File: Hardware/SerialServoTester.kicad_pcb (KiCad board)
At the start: 2 copper layers, 0 parts

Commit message: Update PCB data
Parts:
- added J1: Conn_01x04_Pin, Connector_PinHeader_2.54mm:PinHeader_1x04_P2.54mm_Horizontal, F.Cu at (133.6, 72.4)
- added J2: Screw_Terminal_01x02, TerminalBlock:TerminalBlock_bornier-2_P5.08mm, F.Cu at (123.5, 70.0)
- added P1: USB_C_Plug_USB2.0, Connector_USB:USB_C_Plug_JAE_DX07P024AJ1, F.Cu at (109.0, 77.0)
- added Q1: BSS84, Package_TO_SOT_SMD:SOT-23, F.Cu at (114.9, 72.0)
- added R1: 5.1k, Resistor_SMD:R_0603_1608Metric_Pad0.98x0.95mm_HandSolder, F.Cu at (114.0, 78.0)
- added R2: 5.1k, Resistor_SMD:R_0603_1608Metric_Pad0.98x0.95mm_HandSolder, F.Cu at (120.0, 78.0)
- added R3: 5.1k, Resistor_SMD:R_0603_1608Metric_Pad0.98x0.95mm_HandSolder, F.Cu at (118.0, 72.0)
- added R4: 5.1k, Resistor_SMD:R_0603_1608Metric_Pad0.98x0.95mm_HandSolder, F.Cu at (120.0, 72.1)
- added R5: 5.1k, Resistor_SMD:R_0603_1608Metric_Pad0.98x0.95mm_HandSolder, F.Cu at (118.0, 78.0)
- added R6: 5.1k, Resistor_SMD:R_0603_1608Metric_Pad0.98x0.95mm_HandSolder, F.Cu at (116.0, 78.1)
- added U1: FT230XS, Package_SO:SSOP-16_3.9x4.9mm_P0.635mm, F.Cu at (117.0, 83.0)
- added U2: LT1785AxN8, Package_DIP:DIP-8_W7.62mm, F.Cu at (122.2, 76.2)
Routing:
- net GND: track 0.00 -> 89.1 mm, vias 0 -> 9
- net VCC: track 0.00 -> 65.1 mm, vias 0 -> 3
- net Net-(J1-Pin_4): track 0.00 -> 35.8 mm
- net Net-(U1-TXD): track 0.00 -> 23.3 mm, vias 0 -> 2
- net Net-(P1-D-): track 0.00 -> 21.8 mm
- net Net-(J1-Pin_3): track 0.00 -> 21.3 mm, vias 0 -> 1
- net Net-(U1-RXD): track 0.00 -> 20.9 mm, vias 0 -> 2
- net Net-(P1-CC): track 0.00 -> 20.5 mm
- net Net-(P1-D+): track 0.00 -> 18.7 mm, vias 0 -> 2
- net Net-(U1-CBUS0): track 0.00 -> 17.0 mm, vias 0 -> 2
- net Net-(J1-Pin_2): track 0.00 -> 15.8 mm
- net /~{EN_4PIN}: track 0.00 -> 14.8 mm, vias 0 -> 4
- net Net-(Q1-D): track 0.00 -> 2.76 mm
- added copper zone on B.Cu, net GND
- added copper zone on F.Cu, net VCC
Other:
- board outline added: 39 x 22 mm

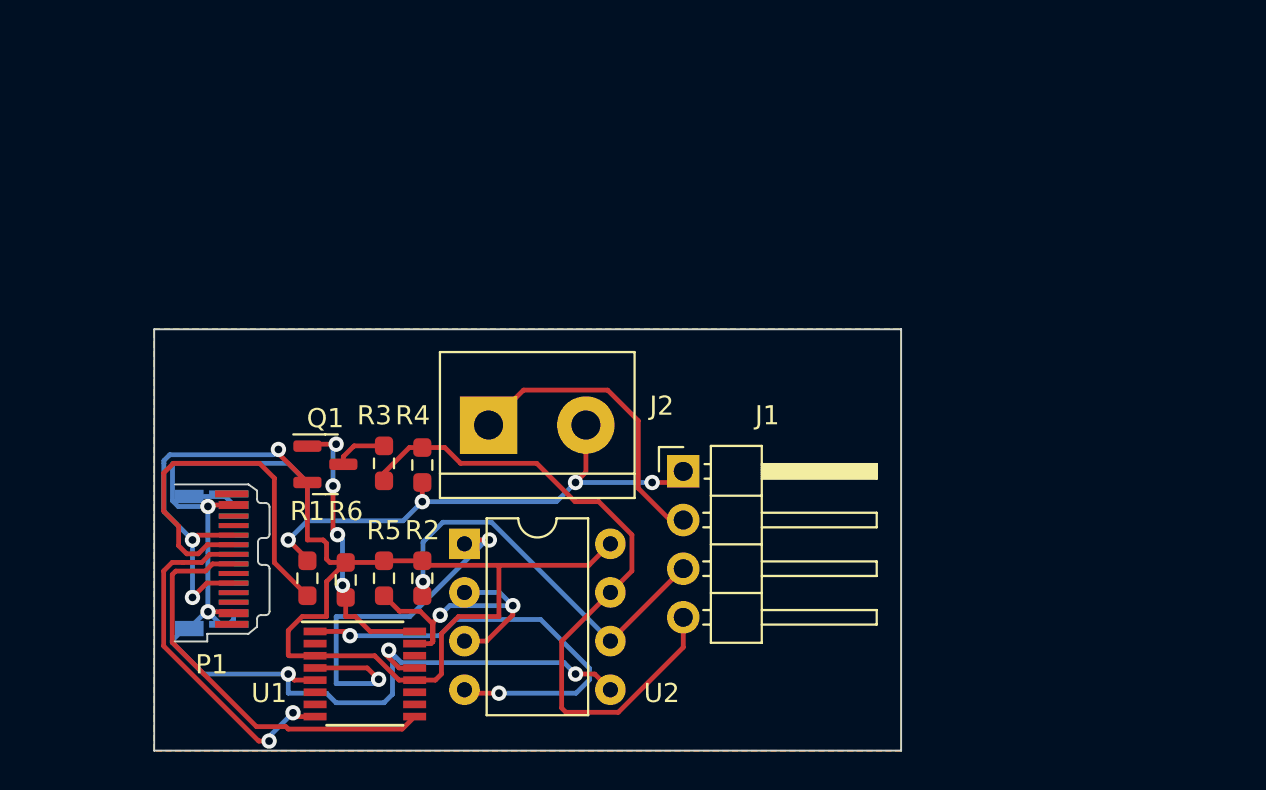
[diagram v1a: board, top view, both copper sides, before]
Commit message: Update PCB design
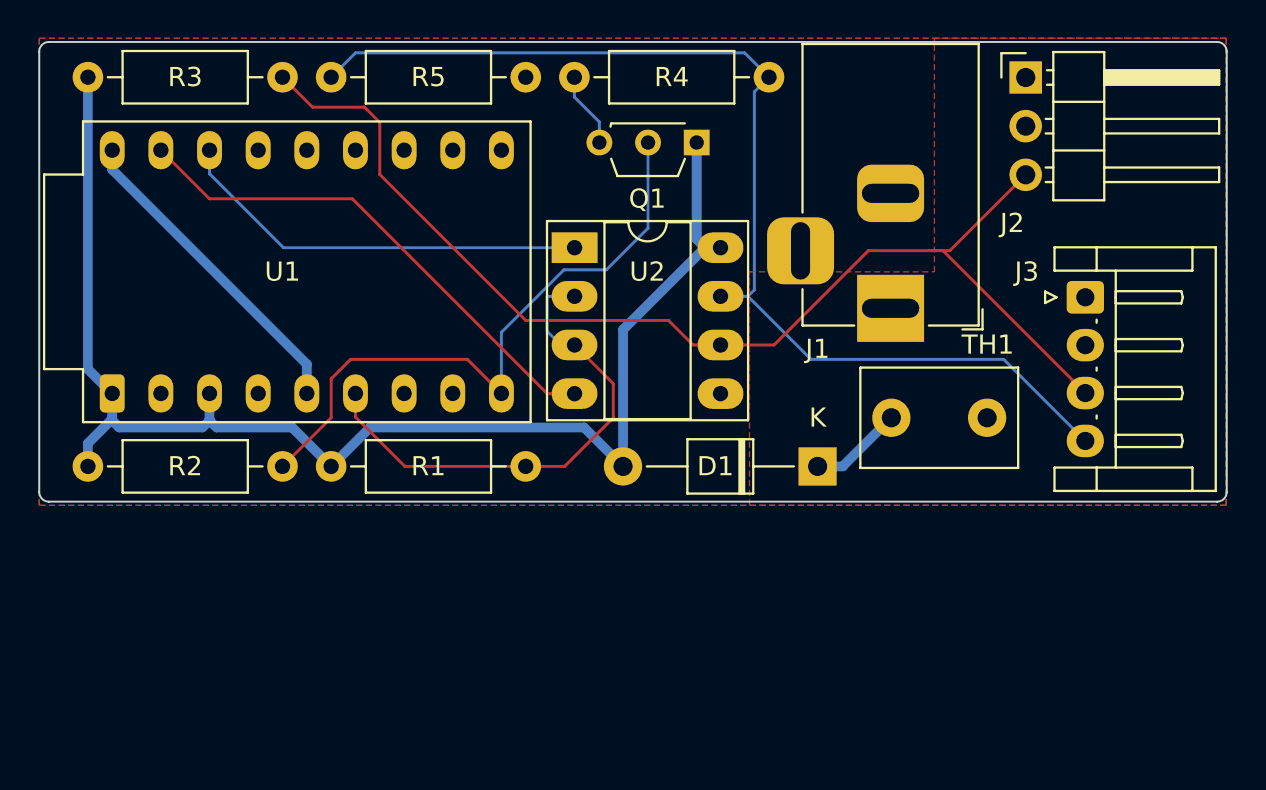
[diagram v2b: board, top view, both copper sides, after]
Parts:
- removed P1: USB_C_Plug_USB2.0, Connector_USB:USB_C_Plug_JAE_DX07P024AJ1
- removed R6: 5.1k, Resistor_SMD:R_0603_1608Metric_Pad0.98x0.95mm_HandSolder
- added D1: 11EQS03L, Diode_THT:D_T-1_P10.16mm_Horizontal, F.Cu at (140.6, 72.2)
- added J3: Conn_01x04_Pin, Connector_JST:JST_EH_S4B-EH_1x04_P2.50mm_Horizontal, F.Cu at (154.6, 63.3)
- added TH1: PTGL07AR820M9A51B0, Capacitor_THT:C_Disc_D8.0mm_W5.0mm_P5.00mm, F.Cu at (149.5, 69.6)
- J1: value Conn_01x04_Pin -> MJ-179PH; footprint Connector_PinHeader_2.54mm:PinHeader_1x04_P2.54mm_Horizontal -> Connector_BarrelJack:BarrelJack_Horizontal
- J2: value Screw_Terminal_01x02 -> Conn_01x03_Pin; footprint TerminalBlock:TerminalBlock_bornier-2_P5.08mm -> Connector_PinHeader_2.54mm:PinHeader_1x03_P2.54mm_Horizontal
- Q1: value BSS84 -> 2SJ498-D; footprint Package_TO_SOT_SMD:SOT-23 -> Package_TO_SOT_THT:TO-92S_Wide
- R1, R2, R3, R4, R5: footprint Resistor_SMD:R_0603_1608Metric_Pad0.98x0.95mm_HandSolder -> Resistor_THT:R_Axial_DIN0207_L6.3mm_D2.5mm_P10.16mm_Horizontal
- U1: value FT230XS -> FT231XS_Breakout; footprint Package_SO:SSOP-16_3.9x4.9mm_P0.635mm -> FootprintLibrary:DIP-18_500_ELL
- U2: footprint Package_DIP:DIP-8_W7.62mm -> Package_DIP:DIP-8_W7.62mm_Socket_LongPads
- moved J2 33.4 mm to (151.5, 51.9)
- moved R5 27.2 mm to (125.4, 51.8), turned to 180 degrees
- moved R4 27.2 mm to (138.1, 51.8), turned to 180 degrees
- moved Q1 25.7 mm to (134.3, 55.2), turned to 180 degrees
- moved U1 21.2 mm to (114.0, 62.0)
- moved R3 20.8 mm to (112.7, 51.8), turned to 180 degrees
- moved U2 16.5 mm to (128.0, 60.7)
- moved J1 13.8 mm to (144.4, 63.9), turned to -90 degrees
- moved R1 12.8 mm to (125.4, 72.2), turned to 180 degrees
- moved R2 9.35 mm to (112.7, 72.2), turned to 180 degrees
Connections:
- J1 pad 1: GND -> VCC
- J1 pad 2: Net-(J1-Pin_2) -> GND
- J1 pad 3: Net-(J1-Pin_3) -> GND
- J2 pad 1: Net-(J1-Pin_2) -> GND
- J2 pad 2: GND -> VCC
- Q1 pad 1: /~{EN_4PIN} -> Net-(D1-A)
- Q1 pad 2: VCC -> /~{EN_4PIN}
- Q1 pad 3: Net-(Q1-D) -> Net-(Q1-S)
- R1 pad 1: Net-(P1-CC) -> Net-(U1-CBUS0)
- R1 pad 2: GND -> Net-(D1-A)
- R2 pad 1: Net-(J1-Pin_3) -> /~{EN_4PIN}
- R2 pad 2: VCC -> Net-(D1-A)
- R3 pad 1: Net-(J1-Pin_4) -> /RS485A
- R3 pad 2: Net-(Q1-D) -> Net-(D1-A)
- R4 pad 1: GND -> /RS485B
- R4 pad 2: Net-(J1-Pin_4) -> Net-(Q1-S)
- R5 pad 1: Net-(U1-CBUS0) -> GND
- R5 pad 2: VCC -> /RS485B
- U1 pad 1: Net-(U1-TXD) -> Net-(D1-A)
- U1 pad 12: VCC -> unconnected-(U1-~{CTS}-Pad12)
- U1 pad 13: GND -> unconnected-(U1-~{RTS}-Pad13)
- U1 pad 14: /LED_TX -> unconnected-(U1-~{DSR}-Pad14)
- U1 pad 15: Net-(U1-CBUS0) -> unconnected-(U1-~{DTR}-Pad15)
- U1 pad 16: /~{EN_4PIN} -> Net-(U1-RXD)
- U1 pad 3: VCC -> Net-(D1-A)
- U1 pad 4: Net-(U1-RXD) -> unconnected-(U1-~{RESET}-Pad4)
- U1 pad 6: unconnected-(U1-~{CTS}-Pad6) -> Net-(U1-CBUS0)
- U1 pad 7: /LED_RX -> unconnected-(U1-CBUS1-Pad7)
- U1 pad 8: Net-(P1-D+) -> unconnected-(U1-CBUS2-Pad8)
- U1 pad 9: Net-(P1-D-) -> /~{EN_4PIN}
- U2 pad 6: Net-(J1-Pin_3) -> /RS485A
- U2 pad 7: Net-(J1-Pin_4) -> /RS485B
- U2 pad 8: VCC -> Net-(D1-A)
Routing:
- net GND: track 89.1 -> 16.9 mm, vias 9 -> 0
- net Net-(D1-A): track 0.00 -> 72.2 mm
- net VCC: track 65.1 -> 0.00 mm, vias 3 -> 0
- net /RS485A: track 0.00 -> 61.1 mm
- net /RS485B: track 0.00 -> 58.0 mm
- net Net-(J1-Pin_4): track 35.8 -> 0.00 mm
- net Net-(P1-D-): track 21.8 -> 0.00 mm
- net Net-(J1-Pin_3): track 21.3 -> 0.00 mm, vias 1 -> 0
- net Net-(P1-CC): track 20.5 -> 0.00 mm
- net Net-(P1-D+): track 18.7 -> 0.00 mm, vias 2 -> 0
- net /~{EN_4PIN}: track 14.8 -> 33.2 mm, vias 4 -> 0
- net Net-(J1-Pin_2): track 15.8 -> 0.00 mm
- net Net-(U1-CBUS0): track 17.0 -> 26.4 mm, vias 2 -> 0
- net Net-(D1-K): track 0.00 -> 4.90 mm
- net Net-(Q1-S): track 0.00 -> 3.95 mm
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- added copper zone on F.Cu, net GND
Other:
- board size 39 x 22 mm -> 62 x 24 mm
